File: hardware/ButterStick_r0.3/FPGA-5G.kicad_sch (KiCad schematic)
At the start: 1 part, among them U4 ECP5UM5G_85_CABGA381

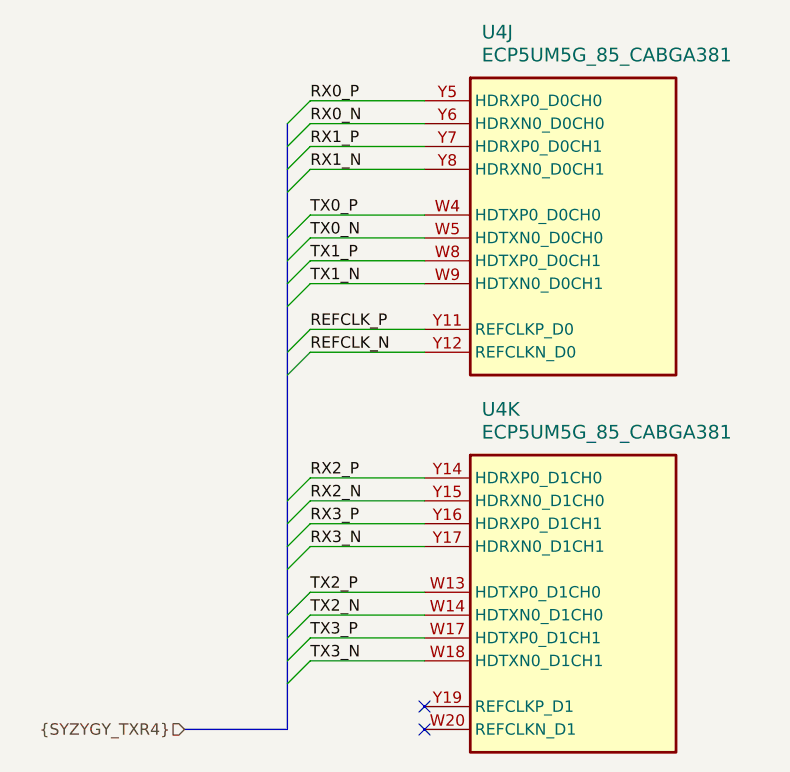
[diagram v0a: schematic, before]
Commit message: hw.r0d3: Tweaking routing
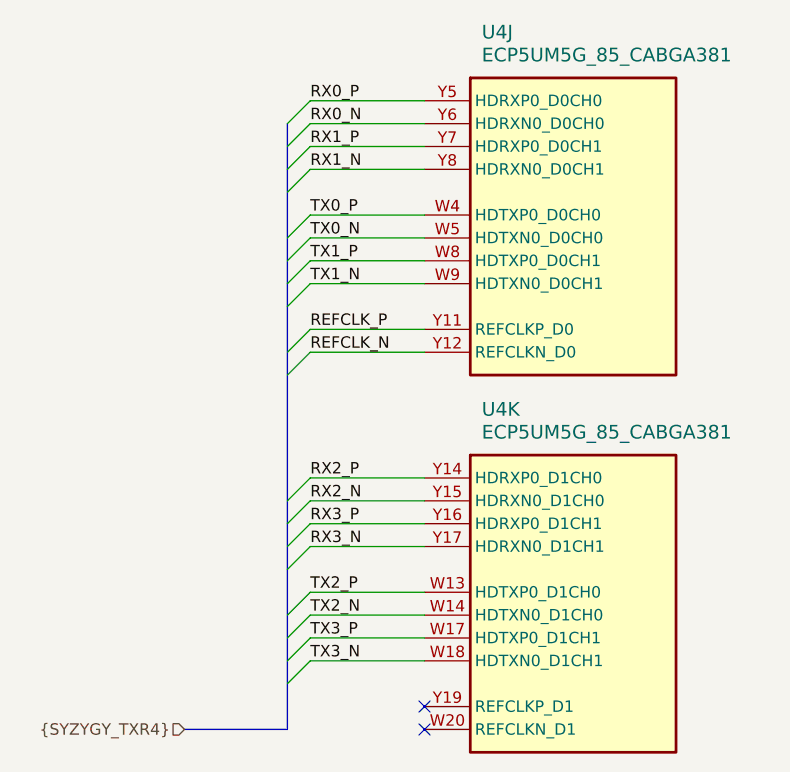
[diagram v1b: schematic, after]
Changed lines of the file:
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@@
 (kicad_sch (version 20200618) (host eeschema "5.99.0-unknown-73168a9~101~ubuntu18.04.1")
-  (page 1 19)
+  (page 11 19)
   (paper "A4")
   (no_connect (at 119.38 132.08))
@@
     (stroke (width 0) (type solid) (color 0 0 0 0))
   )
-  (bus (pts (xy 104.14 85.09) (xy 104.14 92.71))
+  (bus (pts (xy 104.14 85.09) (xy 104.14 87.63))
     (stroke (width 0) (type solid) (color 0 0 0 0))
   )
-  (bus (pts (xy 104.14 92.71) (xy 104.14 109.22))
+  (bus (pts (xy 104.14 87.63) (xy 104.14 95.25))
     (stroke (width 0) (type solid) (color 0 0 0 0))
   )
-  (bus (pts (xy 104.14 109.22) (xy 104.14 114.3))
+  (bus (pts (xy 104.14 95.25) (xy 104.14 111.76))
     (stroke (width 0) (type solid) (color 0 0 0 0))
   )
-  (bus (pts (xy 104.14 114.3) (xy 104.14 121.92))
+  (bus (pts (xy 104.14 111.76) (xy 104.14 116.84))
     (stroke (width 0) (type solid) (color 0 0 0 0))
   )
-  (bus (pts (xy 104.14 121.92) (xy 104.14 124.46))
+  (bus (pts (xy 104.14 116.84) (xy 104.14 124.46))
     (stroke (width 0) (type solid) (color 0 0 0 0))
   )
-  (bus (pts (xy 104.14 124.46) (xy 104.14 129.54))
+  (bus (pts (xy 104.14 124.46) (xy 104.14 127))
     (stroke (width 0) (type solid) (color 0 0 0 0))
   )
-  (bus (pts (xy 104.14 129.54) (xy 104.14 134.62))
+  (bus (pts (xy 104.14 127) (xy 104.14 134.62))
     (stroke (width 0) (type solid) (color 0 0 0 0))
   )
